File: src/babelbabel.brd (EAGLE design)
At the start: 41 x 75.5 mm, 144 parts, among them CON1 CON-4P-TABS-JST_GH-RA, CON10 CON-6P-SM06B, CON101 PINHEAD_1X04-2.54, CON102 PINHEAD_1X03-2.54, CON11 PINHEAD_1X04-2.54, CON12 PINHEAD_1X06-2.54, CON15 PINHEAD_1X04-2.54, CON16 CON-4P-TABS-JST_GH-RA, CON2 PINHEAD_1X04-2.54, CON201 PINHEAD_1X04-2.54, CON202 PINHEAD_1X03-2.54, CON3 PINHEAD_1X04-2.54, CON4 USB-AA-PTH, CON5 CON-4P-TABS-JST_GH-RA, CON6 CON-4P-TABS-JST_GH-RA, CON7 USB-1, IC101 STM32F373CBT6-LQFP48, IC102 STM32F373RCT6, IC103 AP2127-3.3, IC105 TJA1051-SO8, IC108 TPD3S014DBVR-SOT23-6, IC13 STM32F103CBT7, IC14 74LVC2T45, IC15 74LVC2T45, IC16 74LVC2T45, IC17 74LVC2T45, IC201 STM32F373CBT6-LQFP48, IC202 STM32F373RCT6, IC203 AP2127-3.3, IC205 TJA1051-SO8, IC208 TPD3S014DBVR-SOT23-6, IC3 AP2127-3.3, IC9 FE1.1S, J1 CONNECTION-SMD, J2 CONNECTION-SMD, Q101 16MHz, Q102 2N7002, Q201 16MHz, Q202 2N7002, Q7 8MHz, Q8 16MHz, Q9 NTZD3152PT1G

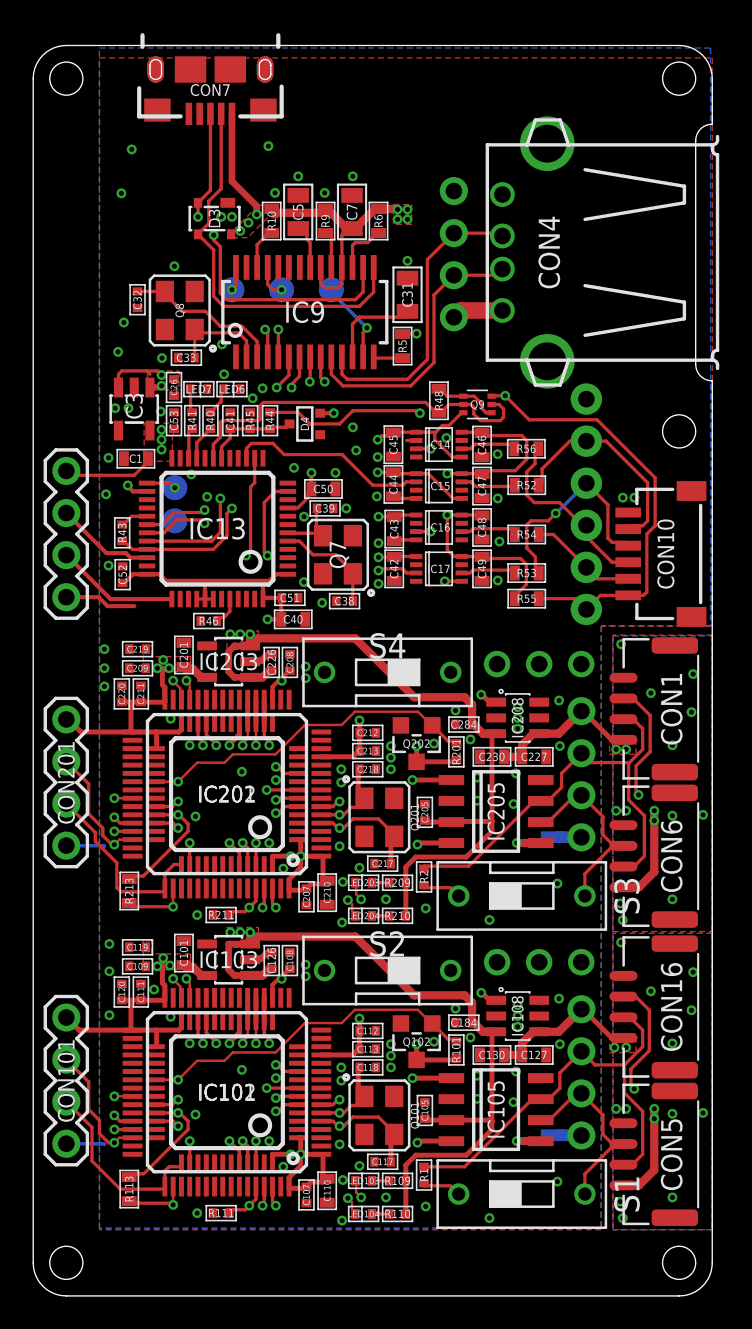
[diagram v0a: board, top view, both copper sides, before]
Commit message: Massive attribute update
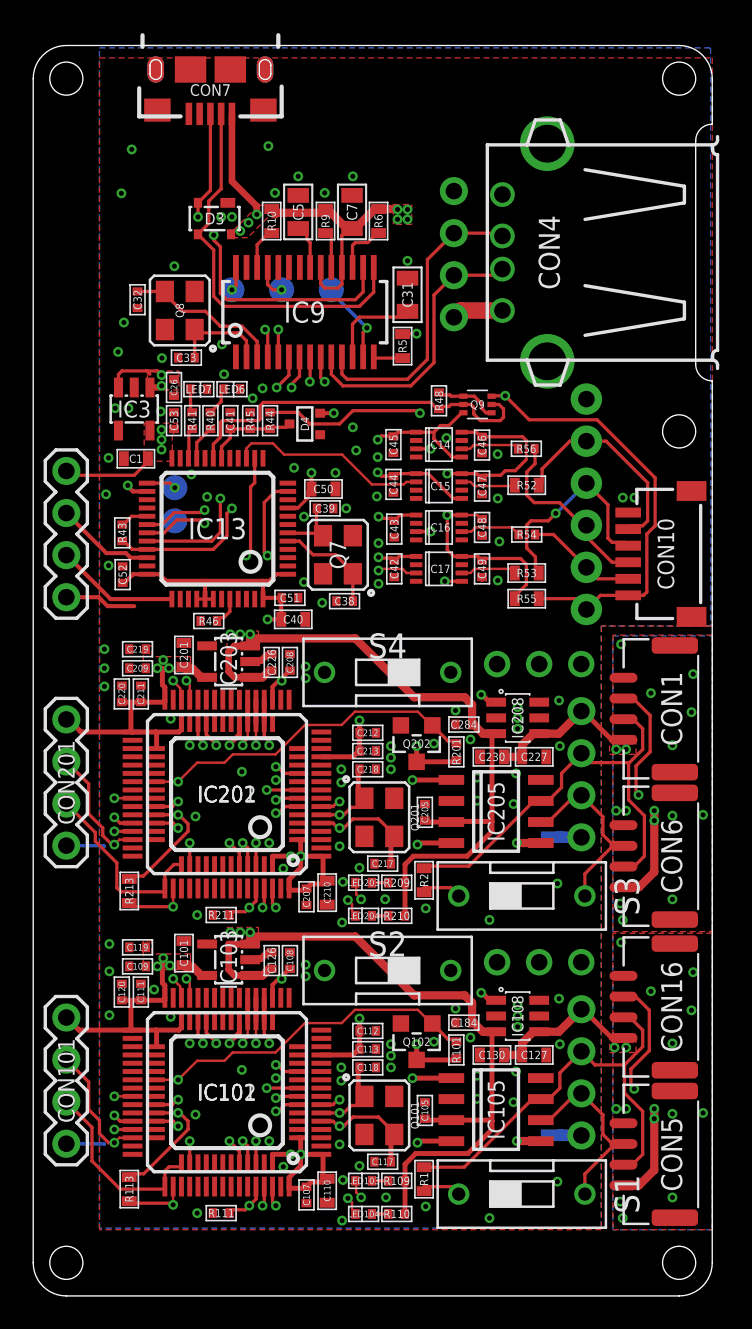
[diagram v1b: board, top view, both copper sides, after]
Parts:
- C1, C40, C50: value 4.7µF -> 4.7uF
- C26: value 1µF -> 1uF
- C32, C33: value 18pF -> 20pF
- C38, C39: value 18pF -> 10pF
- C41, C51, C52, C53: value 0.1µF -> 0.1uF
- C42, C43, C44, C45, C46, C47, C48, C49: value 0.1µF -> 0.1uF; device C_digikey:C0603 -> rc:C0402
- R1, R2: value 100K -> 120R; device rc:R0402 -> rc:R0603
- R48, R54, R56: device R_digikey:R0603 -> rc:R0402
- R52, R53, R55: device R_digikey:R0603 -> rc:R0603
- moved R1 0.25 mm to (23.6, -30.7)
- moved R2 0.20 mm to (23.6, -12.7)
- moved R109 0.05 mm to (21.9, -30.8)
- moved R110 0.05 mm to (21.9, -32.8)
- moved R209 0.05 mm to (21.9, -12.8)
- moved R210 0.05 mm to (21.9, -14.8)
- turned D3 to 270 degrees
- turned IC103 to 0 degrees
- turned IC203 to 0 degrees
- turned IC3 to 90 degrees
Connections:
- net CONSOLE_RX: now also R56.2; no longer R56.P$2
- net CONSOLE_TX: now also R54.2; no longer R54.P$2
- net GND: now also C42.2, C43.2, C44.2, C45.2, C46.1, C47.1, C48.1, C49.1; no longer C42.P$2, C43.P$2, C44.P$2, C45.P$2, C46.P$1, C47.P$1, C48.P$1, C49.P$1
- net N$44: now also R48.1; no longer R48.P$1
- net PWR_BR: now also R48.2; no longer R48.P$2
- net TCK: now also R52.2; no longer R52.P$2
- net TMS: now also R53.2; no longer R53.P$2
- net TPWR: now also R55.2; no longer R55.P$2
- net VDD_3V3: now also C42.1, C43.1, C44.1, C45.1; no longer C42.P$1, C43.P$1, C44.P$1, C45.P$1
- net XRXD: now also R54.1; no longer R54.P$1
- net XTCK: now also R52.1; no longer R52.P$1
- net XTMS: now also R53.1; no longer R53.P$1
- net XTPWR: now also C46.2, C47.2, C48.2, C49.2, R55.1; no longer C46.P$2, C47.P$2, C48.P$2, C49.P$2, R55.P$1
- net XTXD: now also R56.1; no longer R56.P$1
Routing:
- net GND: track 17.9 -> 13.8 mm
- net VDD_3V3: track 82.1 -> 82.6 mm
